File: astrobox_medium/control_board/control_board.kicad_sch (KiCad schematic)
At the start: 63 parts, among them J1 ISP, J2 Output, Q1 BC817, Q10 BC817, Q11 BC817, Q12 BC817, Q13 BC817, Q14 BC817, Q2 BC817, Q3 BC817, Q4 BC817, Q5 BC817, Q6 BC817, Q7 BC817, Q8 BC817, Q9 BC817, SW1 Enable, SW2 Enable PWM, U1 DA56-11EWA, U2 ATmega8535-16A, U3 74LS14

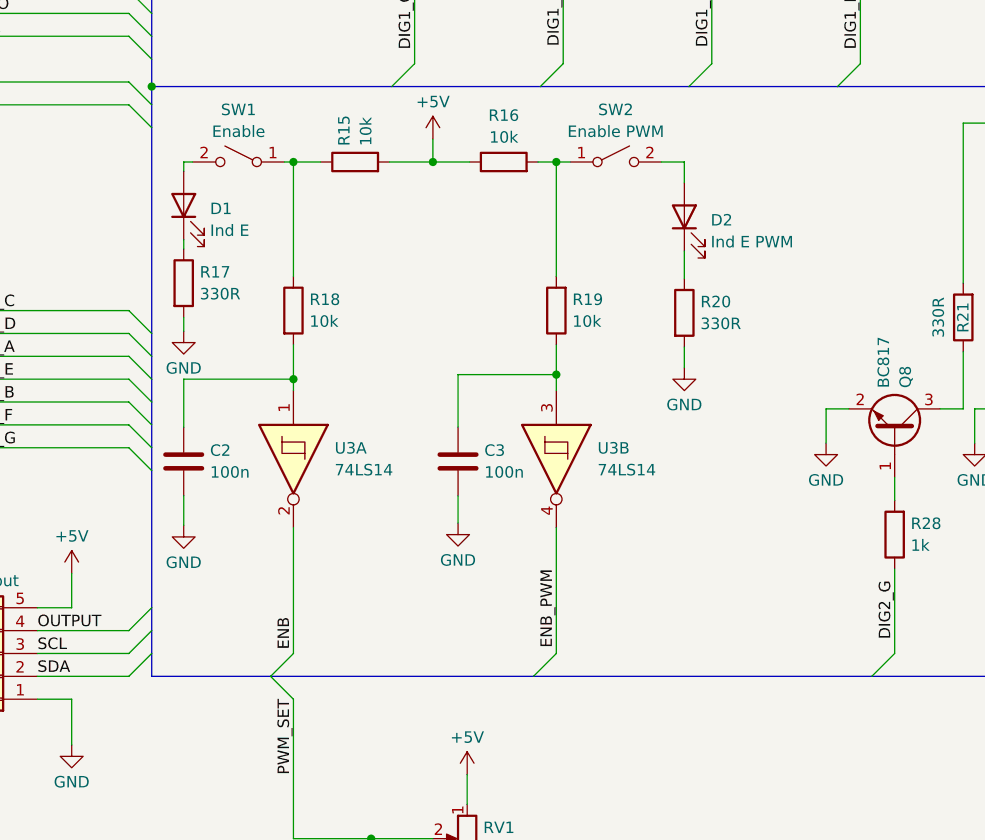
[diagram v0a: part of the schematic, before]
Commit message: Control board update
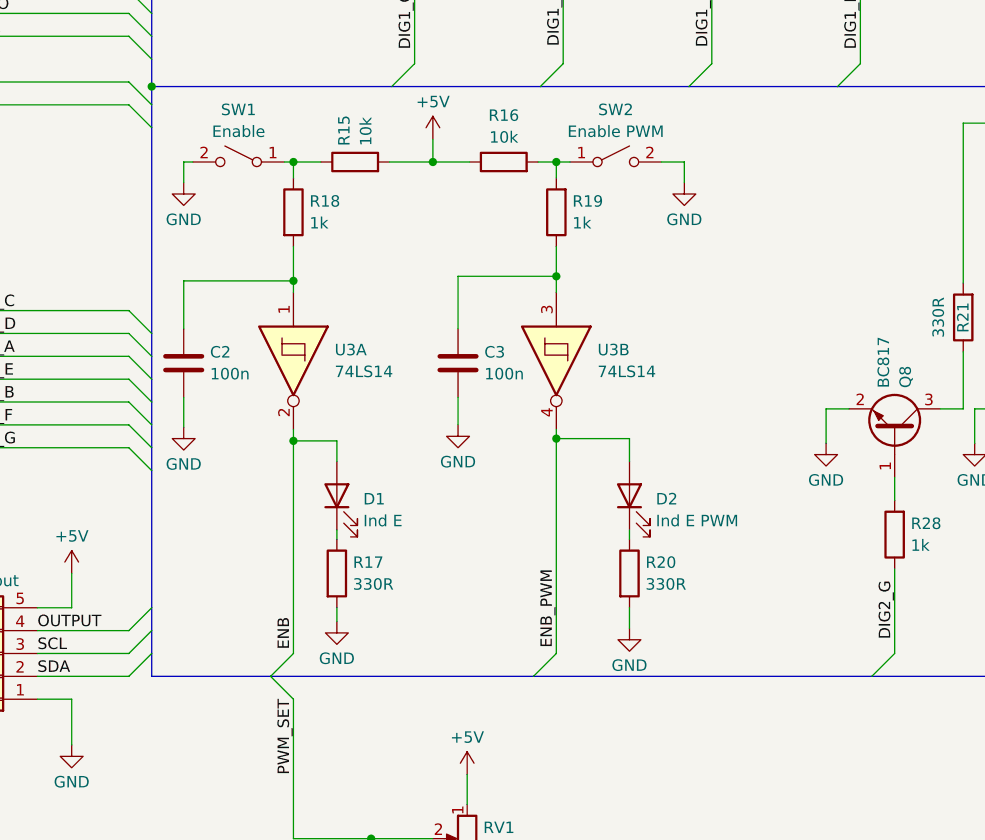
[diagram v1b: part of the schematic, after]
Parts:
- R18, R19: value 10k -> 1k
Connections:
- net ENB: now also D1.2 (A)
- net ENB_PWM: now also D2.2 (A)
- net GND: now also SW1.2 (B), SW2.2 (B)
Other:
- moved on the sheet: C2, C3, D1, D2, R17, R18, R19, R20, U3A, U3B
